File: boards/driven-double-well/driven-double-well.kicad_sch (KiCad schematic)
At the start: 108 parts, among them J1 Conn_01x04, J2 Conn_01x03, J3 Conn_01x02, J4 Conn_01x02, J5 Conn_01x02, J6 Conn_01x03, J7 Conn_01x02, J8 Conn_01x02, Q1 BC560, Q2 BC560, Q3 BC560, Q4 BC560, Q5 BC560, U1 LM13700, U10 TL072, U11 TL072, U12 LM4040LP-10, U13 LM4040LP-10, U2 TL072, U3 MPY634KP, U4 MPY634KP, U5 TL072, U6 LM13700, U7 TL072, U8 LM334Z

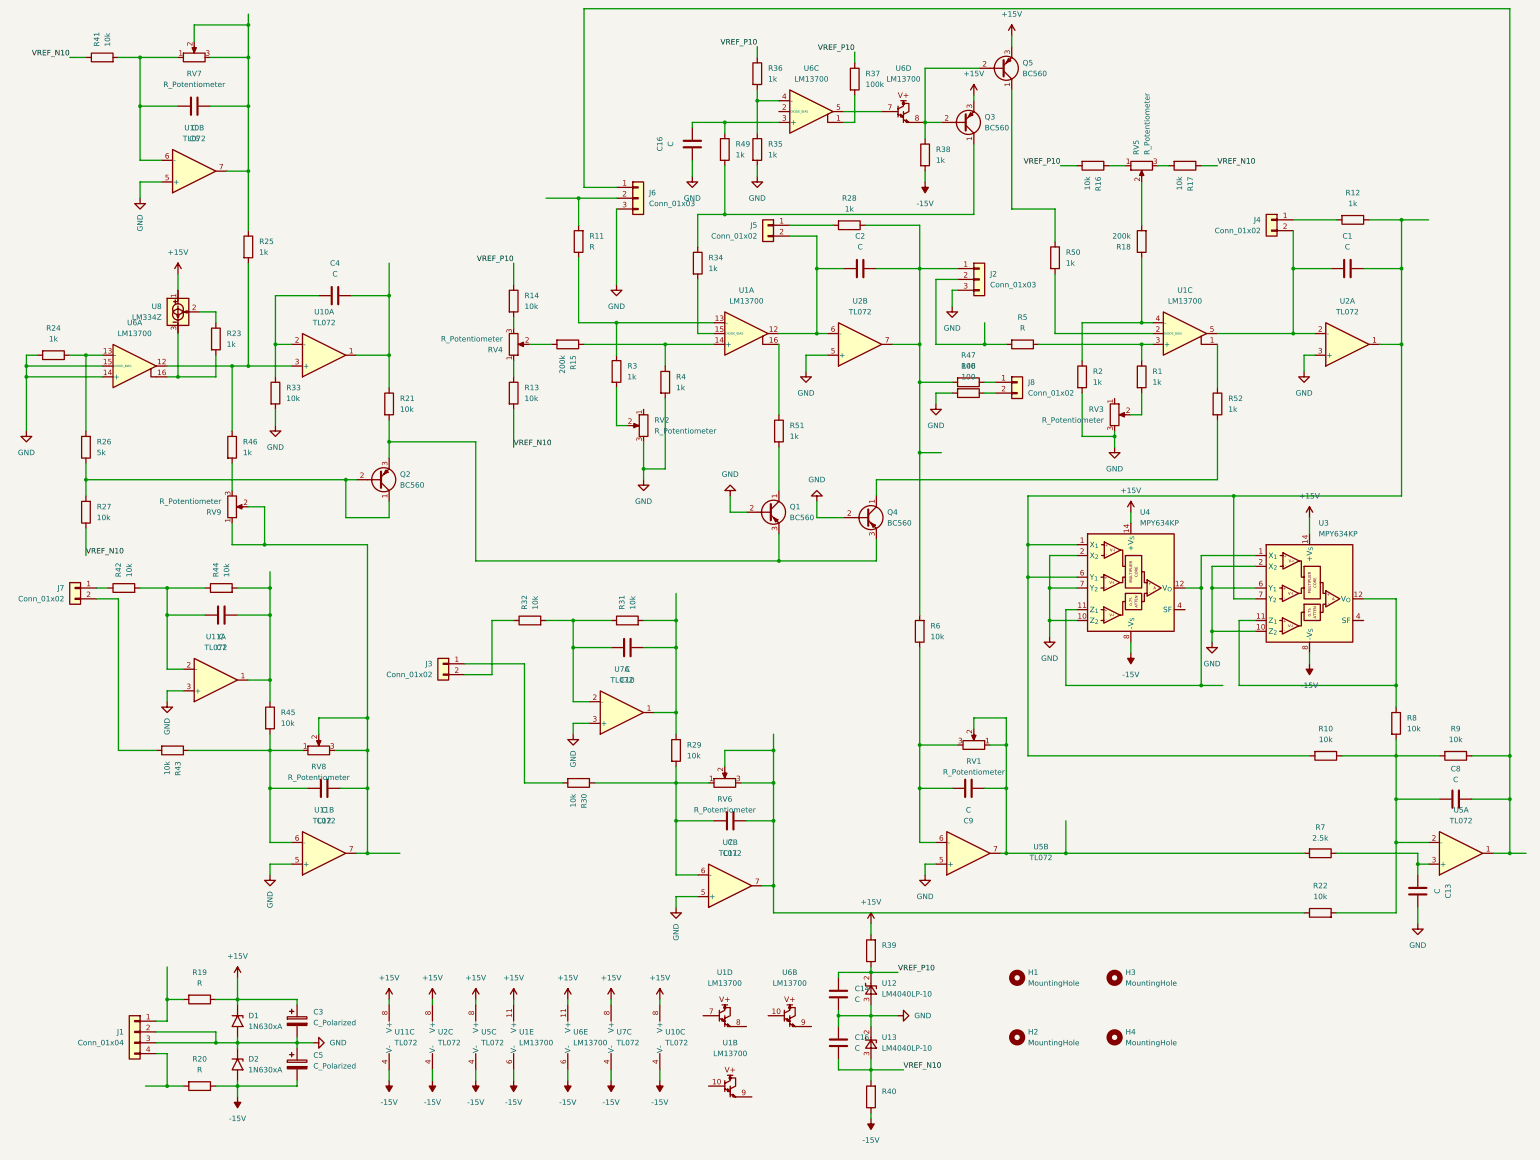
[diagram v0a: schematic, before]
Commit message: Update driven double well board (#2)
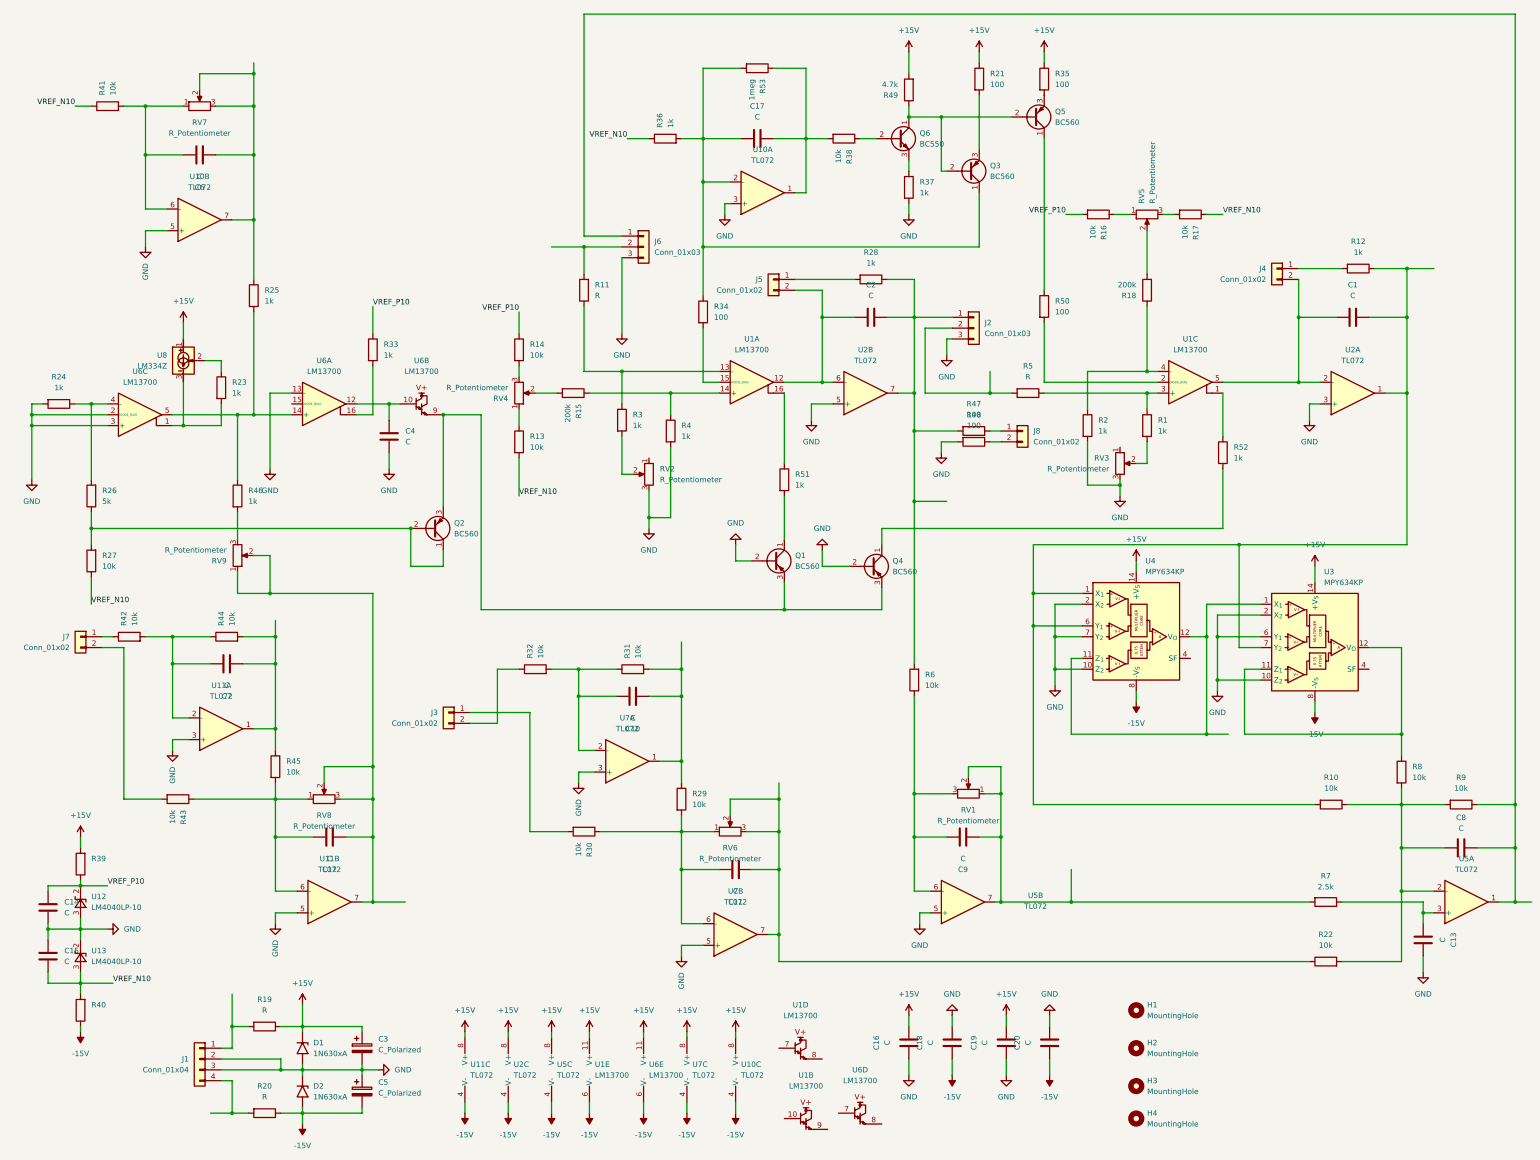
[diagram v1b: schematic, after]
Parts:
- added C17: C, Capacitor_THT:C_Rect_L7.2mm_W4.5mm_P5.00mm_FKS2_FKP2_MKS2_MKP2, symbol Device:C
- added C18, C19, C20: C, Capacitor_THT:C_Disc_D3.4mm_W2.1mm_P2.50mm, symbol Device:C
- added Q6: BC550, Package_TO_SOT_THT:TO-92_HandSolder, symbol Transistor_BJT:BC550
- added R53: 1meg, Resistor_THT:R_Axial_DIN0207_L6.3mm_D2.5mm_P10.16mm_Horizontal, symbol Device:R
- C14, C15: footprint Capacitor_THT:C_Rect_L7.2mm_W4.5mm_P5.00mm_FKS2_FKP2_MKS2_MKP2 -> Capacitor_THT:C_Axial_L12.0mm_D7.5mm_P15.00mm_Horizontal
- C16: footprint Capacitor_THT:C_Rect_L7.2mm_W2.5mm_P5.00mm_FKS2_FKP2_MKS2_MKP2 -> Capacitor_THT:C_Disc_D3.4mm_W2.1mm_P2.50mm
- C4: footprint Capacitor_THT:C_Disc_D3.4mm_W2.1mm_P2.50mm -> Capacitor_THT:C_Axial_L5.1mm_D3.1mm_P10.00mm_Horizontal
- R21: value 10k -> 100
- R33: value 10k -> 1k
- R34, R35, R50: value 1k -> 100
- R37: value 100k -> 1k
- R38: value 1k -> 10k
- R49: value 1k -> 4.7k
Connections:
- net +15V: now also C16.2, R21.1, R35.1, R49.2, C19.2; no longer Q3.3 (E), Q5.3 (E)
- net -15V: now also C18.1, C20.1; no longer R38.2
- net GND: now also C4.2, R37.2, U10.3 (+), U6.13 (-), U6.2 (DIODE_BIAS), U6.3 (+), C18.2, C19.1, C20.2; no longer R33.2, R35.2, U6.14 (+), U6.15 (DIODE_BIAS)
- net VREF_N10: now also R36.1
- net VREF_P10: now also R33.1; no longer R36.1, R37.1
- net at R24.1, R26.2: now also U6.4 (-); no longer U6.13 (-)
- net at Q3.2 (B), Q5.2 (B): now also R49.1, Q6.1 (C); no longer R38.1, U6.8
- net at R25.2, R46.1: now also U6.14 (+), U6.5; no longer U10.3 (+), U6.12
- net at R23.2, U8.3: now also U6.1; no longer U6.16
- net at U6.7: no longer U6.5
- net at Q3.1 (C), R34.1: now also R36.2, U10.2 (-), C17.2, R53.2; no longer R49.2
- net at Q1.3 (E), Q2.3 (E), Q4.3 (E): now also U6.9; no longer R21.2
- net at U6.10: now also C4.1, U6.12
- new net: Q6.2 (B), R38.1
- new net: Q6.3 (E), R37.1
- new net: R33.2, U6.16
- new net: C17.1, R38.2, R53.1, U10.1
- new net: Q5.3 (E), R35.2
- new net: Q3.3 (E), R21.2
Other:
- moved on the sheet: C1, C10, C11, C12, C13, C14, C15, C2, C3, C4, C5, C6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
